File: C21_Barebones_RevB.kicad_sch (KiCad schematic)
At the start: 18 parts, among them J1 Conn_01x02_Pin, J2 TAG_Connect, J3 Conn_01x40_Pin, J4 Conn_01x40_Pin, U1 ATSAMC21N18A-ANT

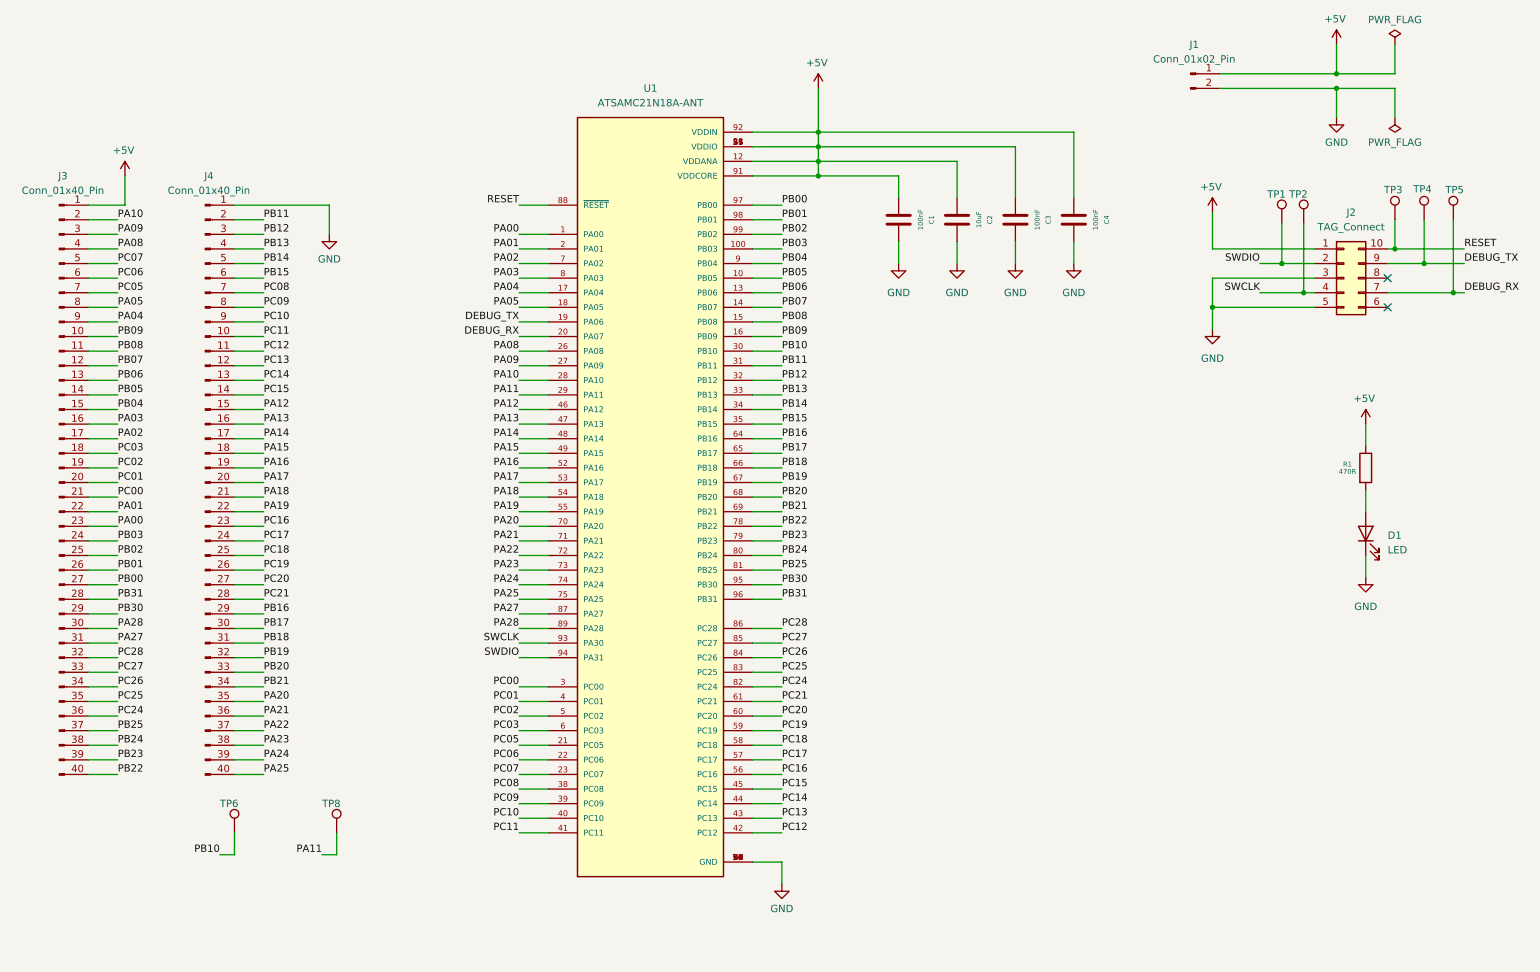
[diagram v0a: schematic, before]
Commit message: Added readme
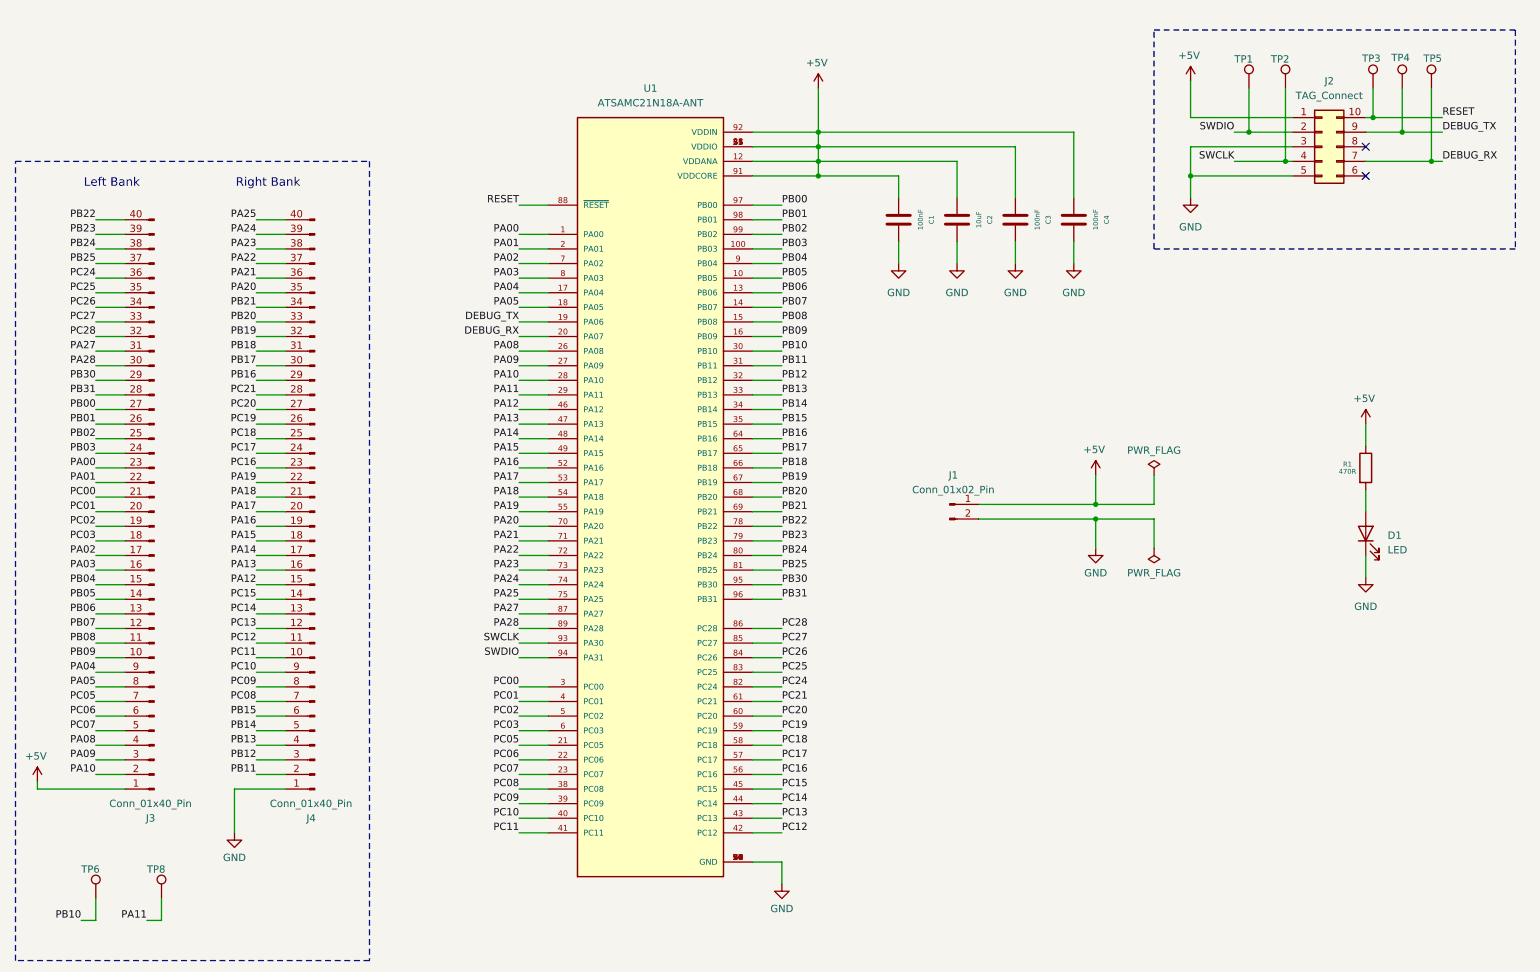
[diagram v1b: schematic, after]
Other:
- note added: "Left Bank"
- note added: "Right Bank"
- moved on the sheet: J1, J2, J3, J4, TP1, TP2, TP3, TP4, TP5, TP6, TP8
